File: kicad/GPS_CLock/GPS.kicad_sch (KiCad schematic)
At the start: 6 parts, among them J401 U.FL, U401 MAX-M10S

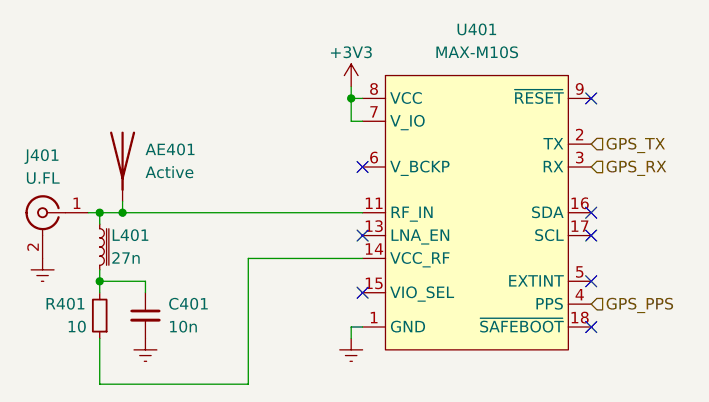
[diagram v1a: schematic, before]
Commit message: update pcb
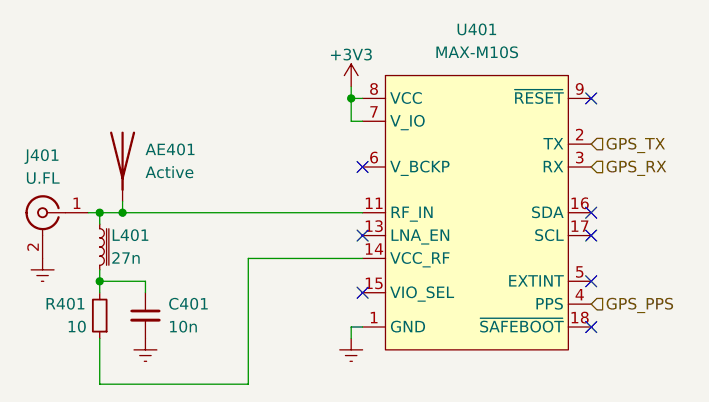
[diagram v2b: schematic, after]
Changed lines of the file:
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@@
   (symbol (lib_id "power:Earth") (at 55.88 57.15 0) (unit 1)
     (in_bom yes) (on_board yes) (fields_autoplaced)
-    (property "Reference" "#PWR0406" (id 0) (at 55.88 63.5 0)
+    (property "Reference" "#PWR0253" (id 0) (at 55.88 63.5 0)
       (effects (font (size 1.27 1.27)) hide)
     )
@@
   (symbol (lib_id "power:Earth") (at 90.17 66.04 0) (unit 1)
     (in_bom yes) (on_board yes) (fields_autoplaced)
-    (property "Reference" "#PWR0409" (id 0) (at 90.17 72.39 0)
+    (property "Reference" "#PWR0254" (id 0) (at 90.17 72.39 0)
       (effects (font (size 1.27 1.27)) hide)
     )
@@
   (symbol (lib_id "power:Earth") (at 67.31 66.04 0) (unit 1)
     (in_bom yes) (on_board yes) (fields_autoplaced)
-    (property "Reference" "#PWR0407" (id 0) (at 67.31 72.39 0)
+    (property "Reference" "#PWR0255" (id 0) (at 67.31 72.39 0)
       (effects (font (size 1.27 1.27)) hide)
     )
@@
   (symbol (lib_id "power:+3V3") (at 90.17 38.1 0) (unit 1)
     (in_bom yes) (on_board yes)
-    (property "Reference" "#PWR0408" (id 0) (at 90.17 41.91 0)
+    (property "Reference" "#PWR0282" (id 0) (at 90.17 41.91 0)
       (effects (font (size 1.27 1.27)) hide)
     )
-    (property "Value" "+3V3" (id 1) (at 90.17 34.29 0))
+    (property "Value" "+3V3" (id 1) (at 90.17 34.544 0))
     (property "Footprint" "" (id 2) (at 90.17 38.1 0)
       (effects (font (size 1.27 1.27)) hide)
